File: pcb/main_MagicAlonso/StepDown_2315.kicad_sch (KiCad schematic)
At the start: 18 parts, among them U5 MP2315, U6 Mini360-MP4560

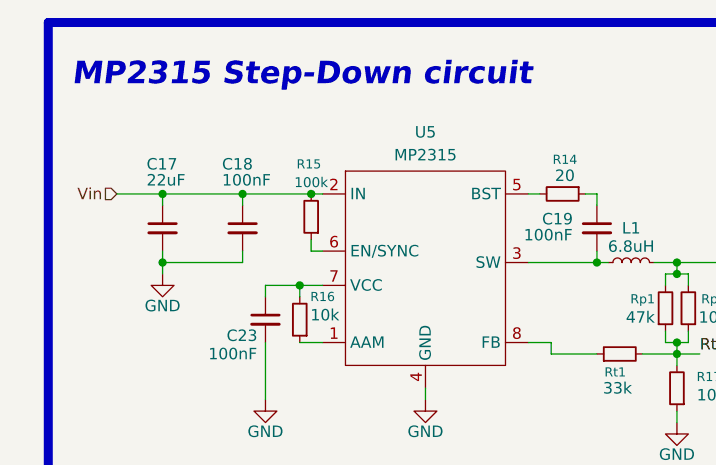
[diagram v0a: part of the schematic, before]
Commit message: some footprint assignment
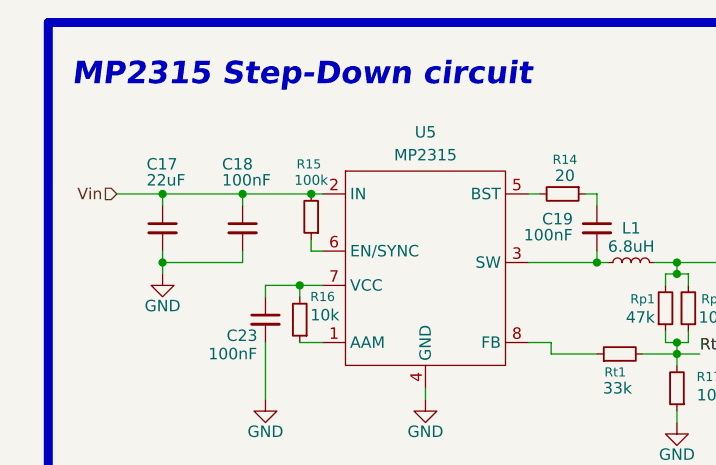
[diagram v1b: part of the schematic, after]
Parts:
- C17, C18, C19, C20, C21, C23: footprint (none) -> Capacitor_SMD:C_0805_2012Metric
- R14, R15, R16, R17, Rp1, Rp2: footprint (none) -> Resistor_SMD:R_0805_2012Metric
- Rt1: footprint (none) -> Resistor_SMD:R_0603_1608Metric
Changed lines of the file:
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@@
 			)
 		)
-		(property "Footprint" ""
+		(property "Footprint" "Resistor_SMD:R_0805_2012Metric"
 			(at 81.28 44.45 0)
 			(effects
@@
 		)
 		(property "Value" "100k"
-			(at 41.91 30.48 0)
+			(at 41.91 30.226 0)
 			(effects
 				(font
@@
 			)
 		)
-		(property "Footprint" ""
+		(property "Footprint" "Resistor_SMD:R_0805_2012Metric"
 			(at 41.91 34.29 0)
 			(effects
@@
 			)
 		)
-		(property "Footprint" ""
+		(property "Footprint" "Resistor_SMD:R_0805_2012Metric"
 			(at 69.85 31.75 0)
 			(effects
@@
 			)
 		)
-		(property "Footprint" ""
+		(property "Footprint" "Capacitor_SMD:C_0805_2012Metric"
 			(at 95.25 43.18 0)
 			(effects
@@
 			)
 		)
-		(property "Footprint" ""
+		(property "Footprint" "Resistor_SMD:R_0603_1608Metric"
 			(at 76.2 49.53 0)
 			(effects
@@
 			)
 		)
-		(property "Footprint" ""
+		(property "Footprint" "Capacitor_SMD:C_0805_2012Metric"
 			(at 36.83 45.72 0)
 			(effects
@@
 			)
 		)
-		(property "Footprint" ""
+		(property "Footprint" "Capacitor_SMD:C_0805_2012Metric"
 			(at 34.29 35.56 0)
 			(effects
@@
 			)
 		)
-		(property "Footprint" ""
+		(property "Footprint" "Capacitor_SMD:C_0805_2012Metric"
 			(at 73.66 35.56 0)
 			(effects
@@
 			)
 		)
-		(property "Footprint" ""
+		(property "Footprint" "Resistor_SMD:R_0805_2012Metric"
 			(at 82.55 53.34 0)
 			(effects
@@
 			)
 		)
-		(property "Footprint" ""
+		(property "Footprint" "Resistor_SMD:R_0805_2012Metric"
 			(at 83.82 44.45 0)
 			(effects
@@
 			)
 		)
-		(property "Footprint" ""
+		(property "Footprint" "Capacitor_SMD:C_0805_2012Metric"
 			(at 25.4 35.56 0)
 			(effects
@@
 			)
 		)
-		(property "Footprint" ""
+		(property "Footprint" "Capacitor_SMD:C_0805_2012Metric"
 			(at 102.87 43.18 0)
 			(effects
@@
 			)
 		)
-		(property "Footprint" ""
+		(property "Footprint" "Resistor_SMD:R_0805_2012Metric"
 			(at 40.64 45.72 0)
 			(effects

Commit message: footprint assingment completed
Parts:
- C22: footprint (none) -> Connector_JST:JST_XH_B2B-XH-A_1x02_P2.50mm_Vertical
- L1: footprint (none) -> Inductor_SMD:L_TDK_SLF6025
- RV1: footprint (none) -> Potentiometer_SMD:Potentiometer_Vishay_TS53YJ_Vertical
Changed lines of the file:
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@@
 			)
 		)
-		(property "Footprint" ""
+		(property "Footprint" "Connector_JST:JST_XH_B2B-XH-A_1x02_P2.50mm_Vertical"
 			(at 110.49 43.18 0)
 			(effects
@@
 			)
 		)
-		(property "Footprint" ""
+		(property "Footprint" "Inductor_SMD:L_TDK_SLF6025"
 			(at 77.47 39.37 0)
 			(effects
@@
 			)
 		)
-		(property "Footprint" ""
+		(property "Footprint" "Potentiometer_SMD:Potentiometer_Vishay_TS53YJ_Vertical"
 			(at 63.5 92.71 0)
 			(effects
